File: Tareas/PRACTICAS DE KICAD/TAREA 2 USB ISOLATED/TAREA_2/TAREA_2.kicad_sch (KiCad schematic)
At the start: 20 parts, among them J1 USB_B, J2 USB_A, U1 ADUM3166BRSZ, U2 B0503S-1WR3_C5444000, X1 3N24000G33YC

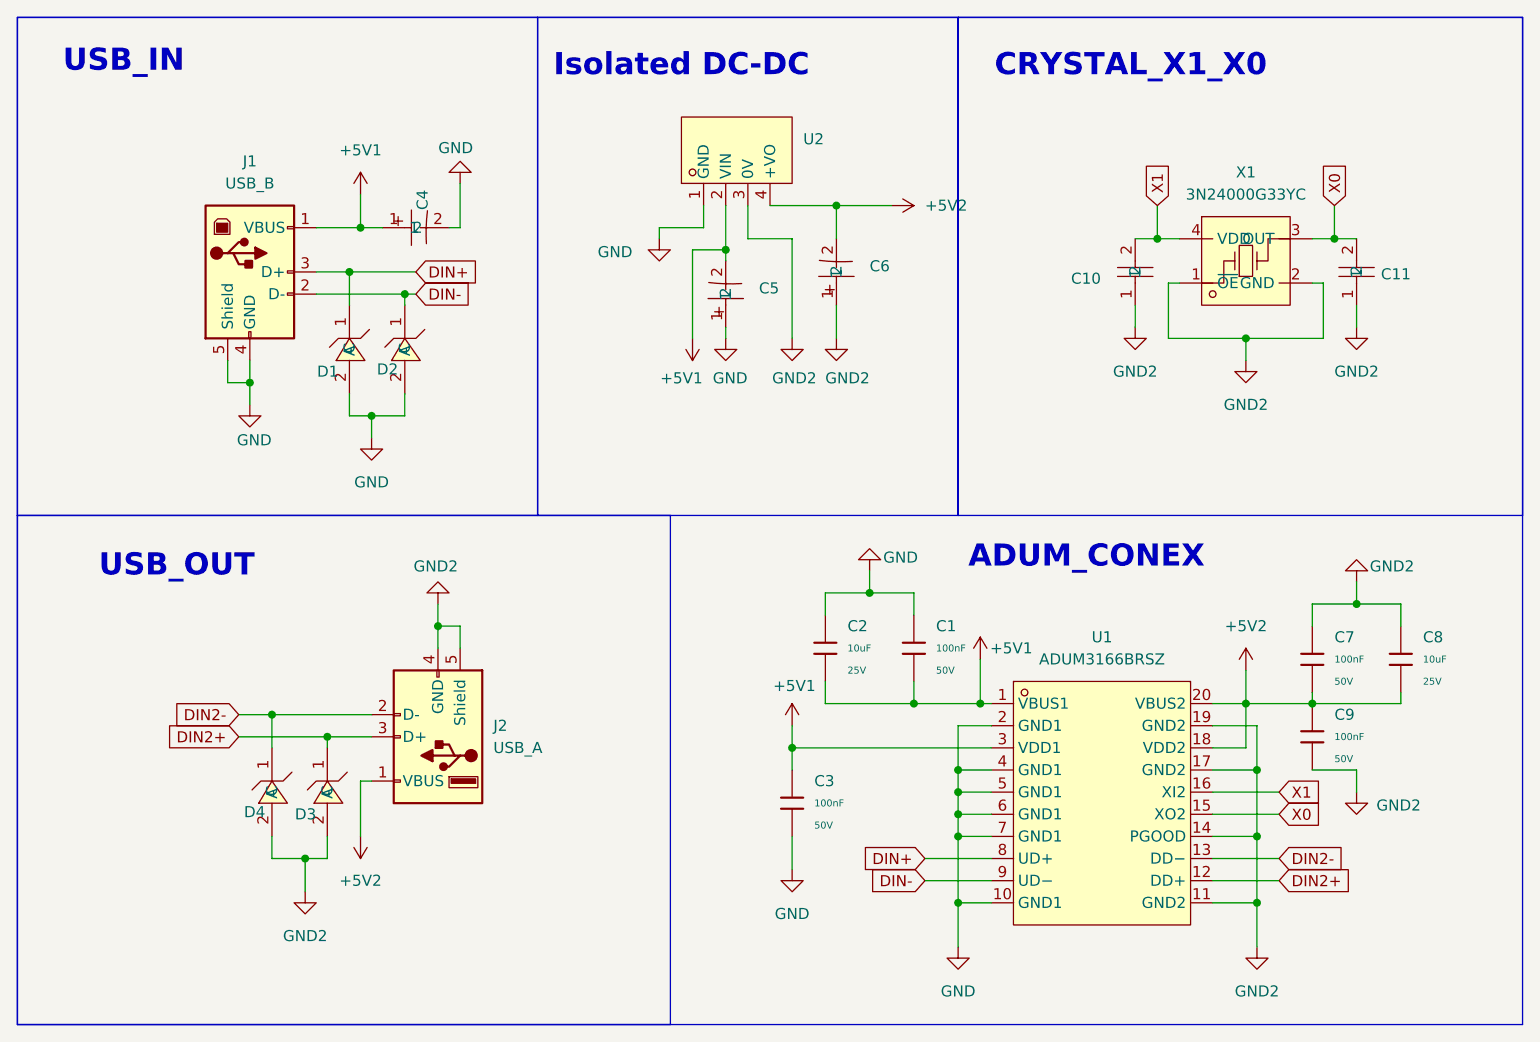
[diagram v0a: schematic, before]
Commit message: LAST UPDATE 5/4/25
USB TERMINADO
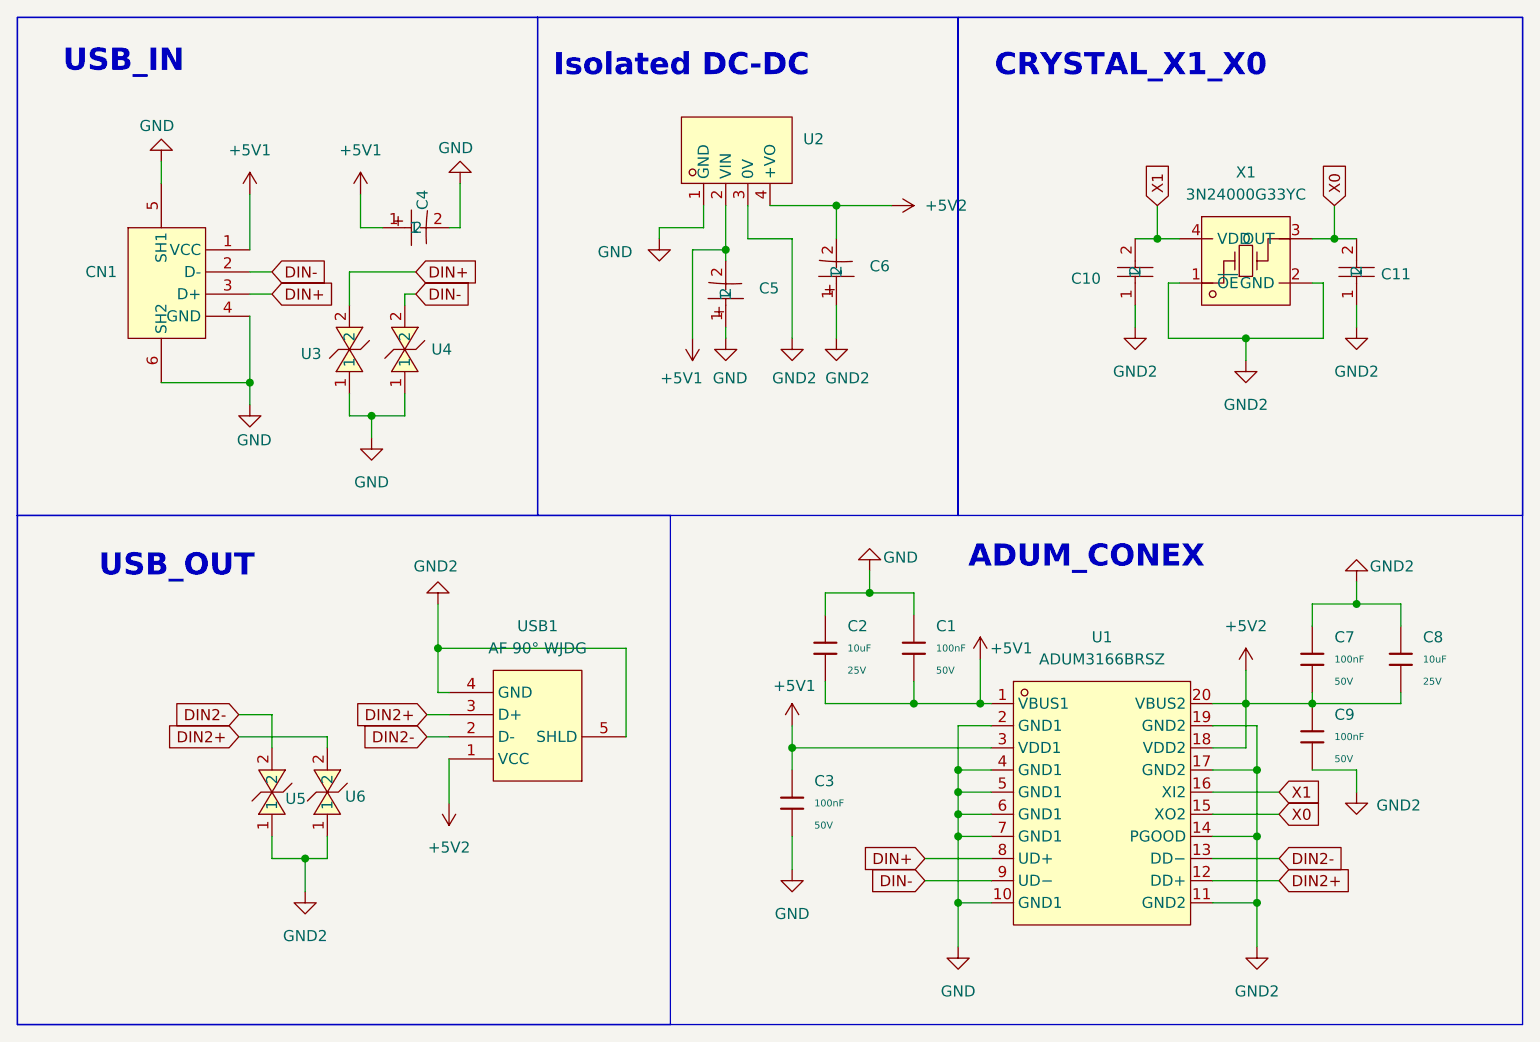
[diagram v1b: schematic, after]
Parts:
- removed D1, D2, D3, D4: SMBJ6.8A, EasyEDA:SMB_L4.6-W3.6-LS5.3-RD, symbol EasyEDA:SMBJ6.8A
- removed J1: USB_B, EasyEDA:USB-B_TH_USB-B-FEMALE-90, symbol Connector:USB_B
- removed J2: USB_A, EasyEDA:USB-A-TH_USB-M-41, symbol Connector:USB_A
- added CN1: USB-B-Female-90, EasyEDA:USB-B_TH_USB-B-FEMALE-90, symbol EasyEDA:USB-B-Female-90
- added U3, U4, U5, U6: TVSS5VCES-02GP-J_C7473318, EasyEDA:SOD-523_L1.2-W0.8-LS1.6-BI, symbol EasyEDA:TVSS5VCES-02GP-J_C7473318
- added USB1: AF 90° WJDG, EasyEDA:USB-A-TH_AF-WJDG, symbol EasyEDA:AF90°WJDG
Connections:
- net +5V1: now also CN1.1 (VCC)
- net +5V2: now also USB1.1 (VCC)
- net DIN+: now also CN1.3 (D+), U3.2
- net DIN-: now also CN1.2 (D-), U4.2
- net DIN2+: now also U6.2, USB1.3 (D+)
- net DIN2-: now also U5.2, USB1.2 (D-)
- net GND: now also CN1.4 (GND), CN1.5 (SH1), CN1.6 (SH2), U3.1, U4.1
- net GND2: now also U5.1, U6.1, USB1.4 (GND), USB1.5 (SHLD)
